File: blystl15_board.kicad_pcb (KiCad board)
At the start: 2 copper layers, 40 x 50 mm, 20 parts, among them J1 SSD1306, J2 Conn_01x03, J3 DOCK_PADS, J4 BNO085, SW2 SW_Push, SW3 SW_Push, SW4 SW_Push, U1 NPM1304-QEAA-R7, U2 MAX30102EFD+T, U3 MAX30208CLB+T

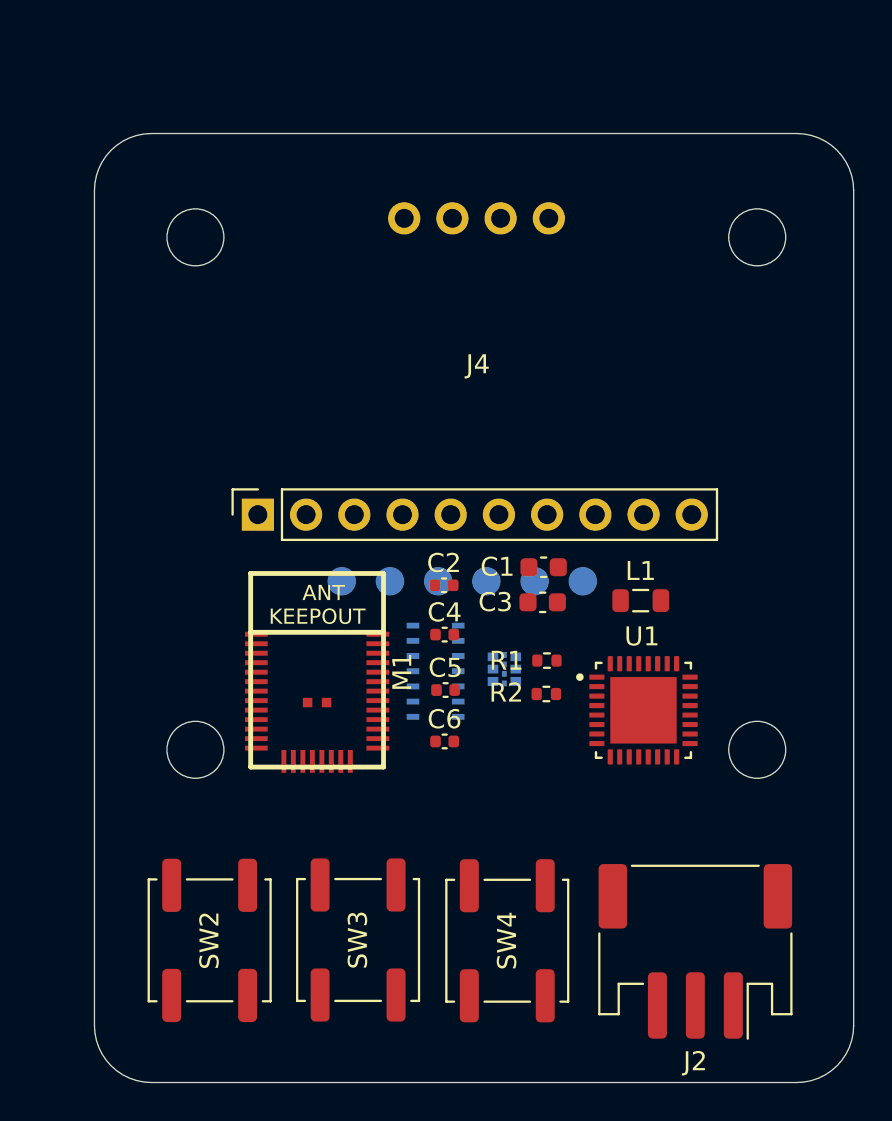
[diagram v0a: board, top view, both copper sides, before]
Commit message: Organized components in pcb layout editor
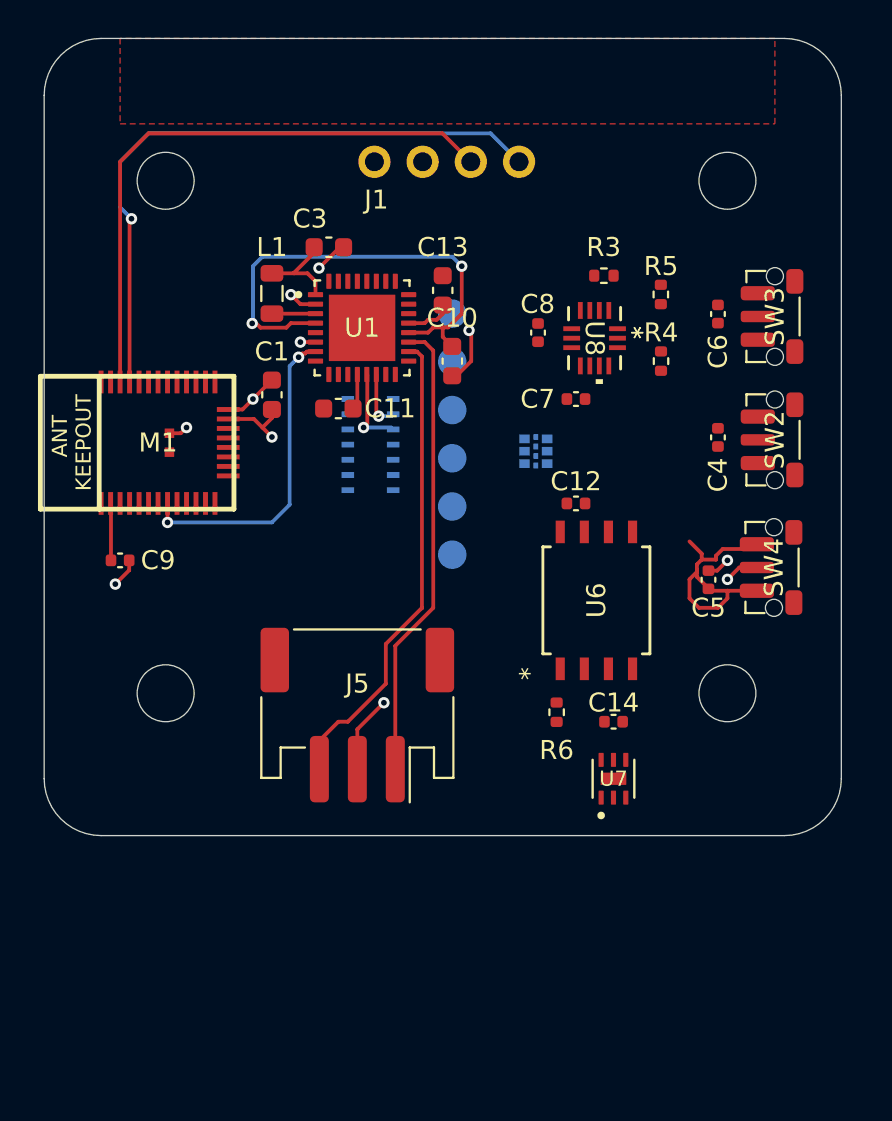
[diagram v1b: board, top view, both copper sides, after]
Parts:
- removed C2: 10000 pF, Capacitor_SMD:C_0402_1005Metric
- removed J2: Conn_01x03, Connector_JST:JST_PH_S3B-PH-SM4-TB_1x03-1MP_P2.00mm_Horizontal
- removed J3: DOCK_PADS, 1_I-SYST_inc:Dock_Pads_6Pin
- removed J4: BNO085, 1_I-SYST_inc:BNO085_Module
- removed R1: 4.7k, Resistor_SMD:R_0402_1005Metric
- removed R2: 4.7K, Resistor_SMD:R_0402_1005Metric
- added C10: 10µF, Capacitor_SMD:C_0603_1608Metric, F.Cu at (152.5, 97.0)
- added C11: 0.1µF, Capacitor_SMD:C_0603_1608Metric, F.Cu at (146.5, 99.5)
- added C12: 0.1 μF, Capacitor_SMD:C_0402_1005Metric, F.Cu at (159.0, 104.5)
- added C13: 1µF, Capacitor_SMD:C_0603_1608Metric, F.Cu at (152.0, 93.3)
- added C14: 0.1 μF, Capacitor_SMD:C_0402_1005Metric, F.Cu at (161.0, 116.0)
- added C7: 0.1 μF, Capacitor_SMD:C_0402_1005Metric, F.Cu at (159.0, 99.0)
- added C8: 0.1 μF, Capacitor_SMD:C_0402_1005Metric, F.Cu at (157.0, 95.5)
- added C9: 0.01 μF, Capacitor_SMD:C_0402_1005Metric, F.Cu at (135.0, 107.5)
- added J5: Conn_01x03, Connector_JST:JST_PH_S3B-PH-SM4-TB_1x03-1MP_P2.00mm_Horizontal, F.Cu at (147.5, 115.7)
- added J6: DOCK_PADS, 1_I_Syst.inc:Dock_Pads_6Pin, B.Cu at (152.5, 100.8)
- added R3: 10kΩ, Resistor_SMD:R_0402_1005Metric, F.Cu at (160.5, 92.5)
- added R4: 4.7kΩ, Resistor_SMD:R_0402_1005Metric, F.Cu at (163.5, 97.0)
- added R5: 4.7kΩ, Resistor_SMD:R_0402_1005Metric, F.Cu at (163.5, 93.5)
- added R6: 10kΩ, Resistor_SMD:R_0402_1005Metric, F.Cu at (158.0, 115.5)
- added U6: W25Q80DVSSIG, 1_I_Syst.inc:WIN_SS-8_WIN-L, F.Cu at (160.1, 109.6)
- added U7: OPT3001DNPRQ1, 1_I_Syst.inc:SON65P200X200X65-7N, F.Cu at (161.0, 119.0)
- added U8: LSM6DSV80X, 1_I_Syst.inc:QFN_LSM6DSV80XTR_STM-M, F.Cu at (160.0, 95.8)
- C4, C5, C6: value 10000 pF -> 0.01 μF
- J1: footprint 1_I-SYST_inc:OLED_1.3in_I2C -> 1_I_Syst.inc:OLED_1.3in_I2C
- M1: value ~ -> BLYSTL15; footprint 1_I-SYST_inc:BLYSTL15 -> 1_I_Syst.inc:BLYSTL15
- SW2, SW3, SW4: footprint Button_Switch_SMD:SW_Push_1P1T_NO_CK_KSC7xxJ -> Button_Switch_SMD:SW_Push_1P1T-MP_NO_Horizontal_Alps_SKRTLAE010
- U1: value NPM1304-QEAA-R7 -> NPM1304; footprint 1_I-SYST_inc:QFN50P500X500X90-33N -> 1_I_Syst.inc:QFN50P500X500X90-33N
- U2: footprint 1_I-SYST_inc:21-1048_F143A5&plus_1_MXM-L -> 1_I_Syst.inc:21-1048_F143A5&plus_1_MXM-L
- U3: footprint 1_I-SYST_inc:21-100265_MXM -> 1_I_Syst.inc:21-100265_MXM
- moved SW2 39.8 mm to (169.5, 101.2)
- moved SW3 39.5 mm to (169.5, 94.7)
- moved C6 26.7 mm to (166.5, 94.5), turned to 90 degrees
- moved L1 25.3 mm to (143.0, 93.4), turned to -90 degrees
- moved U1 25.0 mm to (147.8, 95.2)
- moved SW4 24.2 mm to (169.4, 107.9)
- moved C3 21.8 mm to (146.0, 91.0)
- moved C4 17.8 mm to (166.5, 101.0), turned to 90 degrees
- moved C1 17.0 mm to (143.0, 98.8), turned to 90 degrees
- moved M1 15.5 mm to (137.0, 101.3), turned to 0 degrees
- moved C5 15.0 mm to (166.0, 108.5), turned to 90 degrees
- moved U2 12.4 mm to (148.2, 101.4)
- moved U3 11.6 mm to (156.9, 101.8)
- moved J1 3.37 mm to (152.2, 101.0)
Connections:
- C6 pad 1: /P0.09 -> /P2.00
- SW3 pad 1: /P0.09 -> /P2.00
- U1 pad 18: /NTC -> /Power Management/NTC
- U1 pad 19: /VBAT -> /Power Management/VBAT
- U1 pad 21: /VBUS -> /Power Management/VBUS
- U2 pad 10: /VBAT -> /Sensors/VBAT
- U2 pad 9: /VBAT -> /Sensors/VBAT
- U3 pad 7: /P2.06 -> /P2.03
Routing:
- net /P1.09: track 0.00 -> 38.6 mm, vias 0 -> 2
- net /P1.10: track 0.00 -> 34.4 mm, vias 0 -> 1
- net /Power Management/NTC: track 0.00 -> 25.1 mm
- net Net-(U1-PVDD): track 0.00 -> 24.9 mm, vias 0 -> 2
- net /Power Management/VBAT: track 0.00 -> 24.4 mm
- net GND: track 0.00 -> 19.7 mm, vias 0 -> 10
- net /P2.07: track 0.00 -> 16.8 mm, vias 0 -> 2
- net /P0.03: track 0.00 -> 13.6 mm
- net VDD: track 0.00 -> 10.8 mm, vias 0 -> 1
- net /nRESET: track 0.00 -> 3.01 mm
- net /Power Management/VBUS: track 0.00 -> 2.45 mm
- net Net-(U1-SW1): track 0.00 -> 2.29 mm
- added copper zone on F.Cu, net /Sensors/QVAR_SWIPE
- added copper zone on In1.Cu, net GND
- added copper zone on In2.Cu, net VDD
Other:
- board size 40 x 50 mm -> 42 x 42 mm
- copper layers 2 -> 4
